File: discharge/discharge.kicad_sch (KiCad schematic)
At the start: 23 parts, among them J1 Conn_SDC, J2 Conn_HV_IN, J3 Conn_HV_OUT, J4 GND, J5 Conn_HV_IN, J6 Conn_HV_OUT, J7 Conn, K1 Relay_SPST-NC, K2 Relay_SPST-NC, K3 JY-12H-K, Q2 Si2301CDS, U1 SE555D

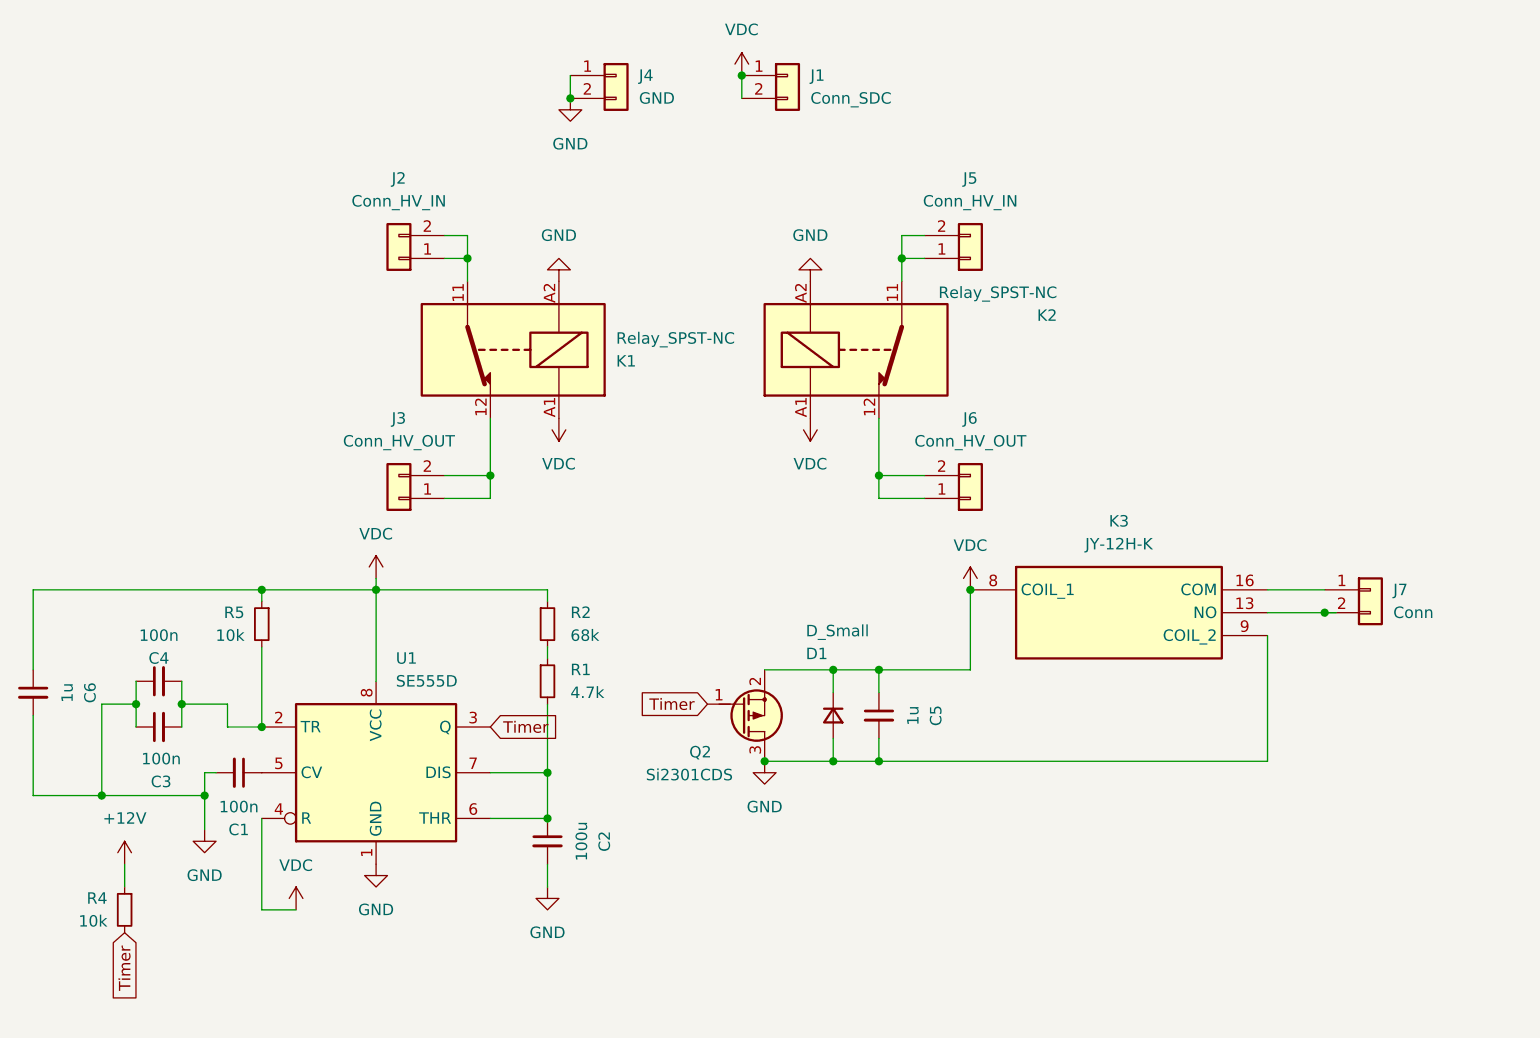
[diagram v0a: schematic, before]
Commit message: modify discharge ver2
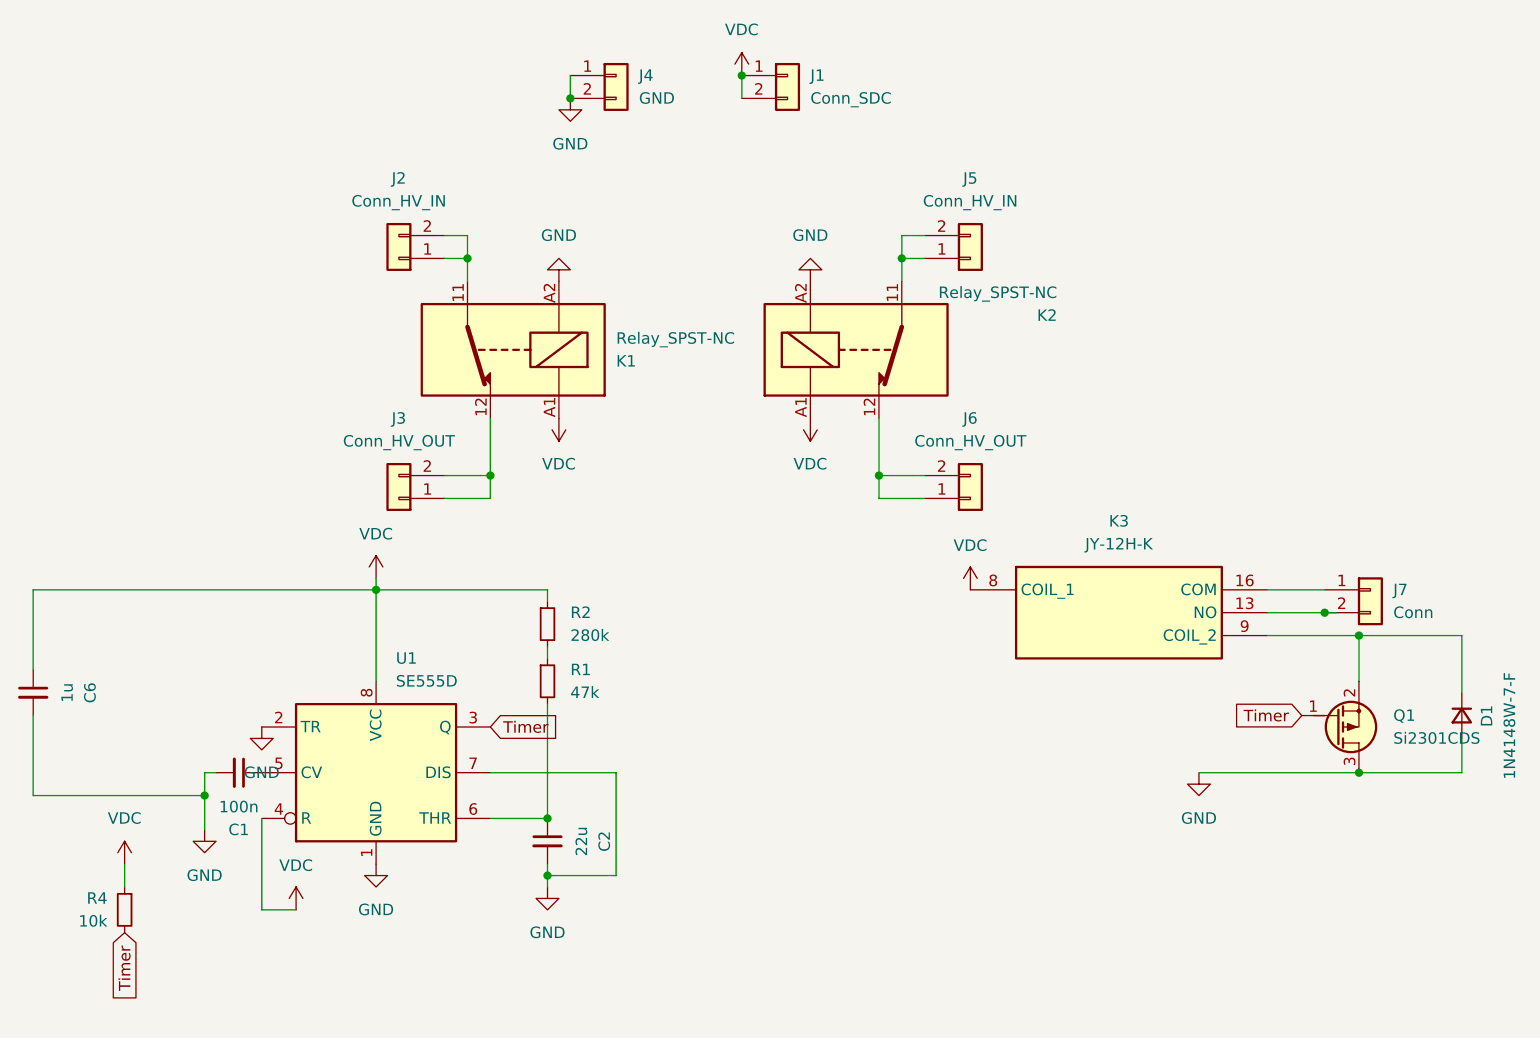
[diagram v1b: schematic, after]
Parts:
- removed C3, C4: 100n, Capacitor_SMD:C_0603_1608Metric, symbol Device:C_Small
- removed C5: 1u, Capacitor_SMD:C_0603_1608Metric, symbol Device:C_Small
- removed Q2: Si2301CDS, Package_TO_SOT_SMD:SOT-23, symbol PCM_Transistor_MOSFET_AKL:Si2301CDS
- removed R5: 10k, Resistor_SMD:R_0603_1608Metric, symbol Device:R_Small
- added Q1: Si2301CDS, Package_TO_SOT_SMD:SOT-23, symbol PCM_Transistor_MOSFET_AKL:Si2301CDS
- C2: value 100u -> 22u; footprint Capacitor_SMD:C_0603_1608Metric -> Capacitor_SMD:C_0805_2012Metric
- D1: value D_Small -> 1N4148W-7-F
- R1: value 4.7k -> 47k
- R2: value 68k -> 280k
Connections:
- net +12V is gone; now on net VDC: R4.1
- net GND: now also U1.2 (TR), U1.7 (DIS), Q1.3 (D); no longer K3.9 (COIL_2)
- net Timer: now also Q1.1 (G)
- net VDC: no longer D1.1 (K)
- net at C2.1, R1.2, U1.6 (THR): no longer U1.7 (DIS)
- new net: D1.1 (K), K3.9 (COIL_2), Q1.2 (S)
